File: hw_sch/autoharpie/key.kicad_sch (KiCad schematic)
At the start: 32 parts

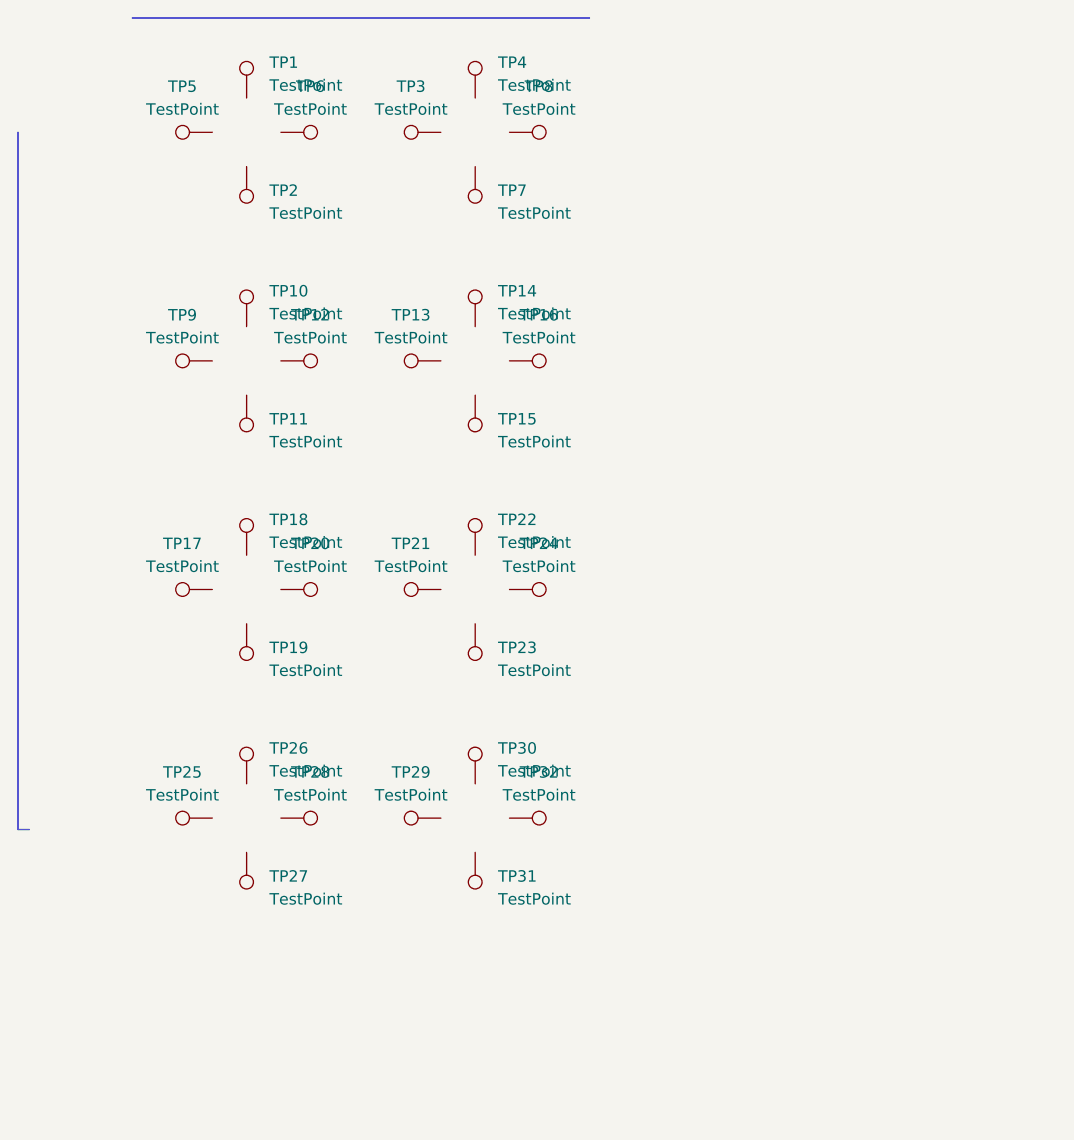
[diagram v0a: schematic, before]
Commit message: DAC, touch sensors
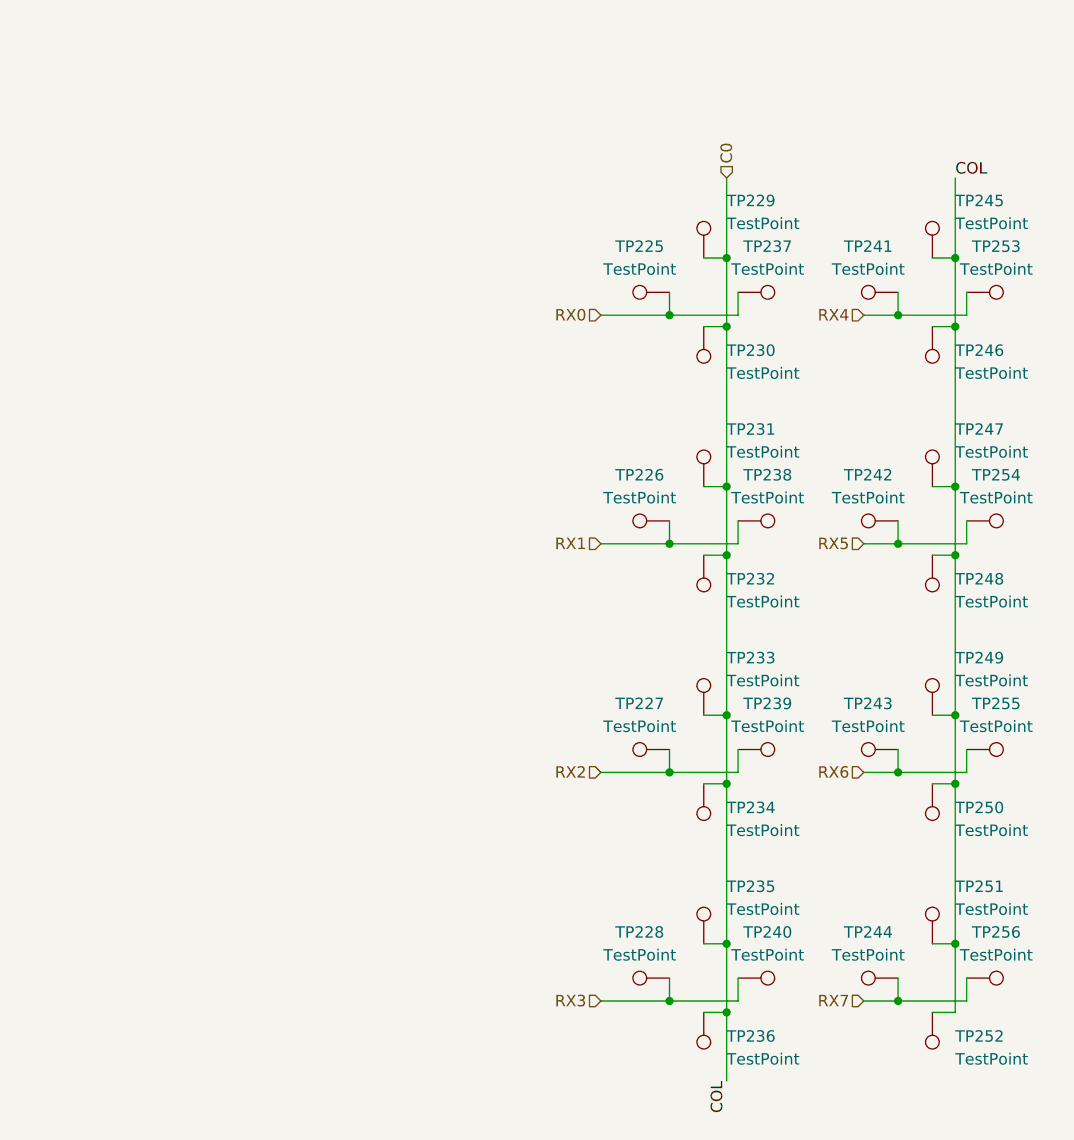
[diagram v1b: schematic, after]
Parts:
- renumbered TP5 to TP225, TP9 to TP226, TP17 to TP227, TP25 to TP228, TP1 to TP229, TP2 to TP230, TP10 to TP231, TP11 to TP232, TP18 to TP233, TP19 to TP234, TP26 to TP235, TP27 to TP236, TP6 to TP237, TP12 to TP238, TP20 to TP239, TP28 to TP240, TP3 to TP241, TP13 to TP242, TP21 to TP243, TP29 to TP244, TP4 to TP245, TP7 to TP246, TP14 to TP247, TP15 to TP248, TP22 to TP249, TP23 to TP250, TP30 to TP251, TP31 to TP252, TP8 to TP253, TP16 to TP254, TP24 to TP255, TP32 to TP256
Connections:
- net RX0: now reaches TP225.1
- net RX0: now also TP237.1
- net RX6: now reaches TP243.1
- net RX6: now also TP255.1
- net RX7: now reaches TP256.1
- net RX7: now also TP244.1
- net C0: now reaches TP235.1
- net C0: now also TP229.1, TP230.1, TP231.1, TP232.1, TP233.1, TP234.1, TP236.1, TP245.1, TP246.1, TP247.1, TP248.1, TP249.1, TP250.1, TP251.1, TP252.1
- net RX3: now reaches TP228.1
- net RX3: now also TP240.1
- net RX1: now reaches TP238.1
- net RX1: now also TP226.1
- net RX2: now reaches TP239.1
- net RX2: now also TP227.1
- net RX5: now reaches TP242.1
- net RX5: now also TP254.1
- net RX4: now reaches TP253.1
- net RX4: now also TP241.1
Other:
- moved on the sheet: TP225, TP226, TP227, TP228, TP229, TP230, TP231, TP232, TP233, TP234, TP235, TP236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
